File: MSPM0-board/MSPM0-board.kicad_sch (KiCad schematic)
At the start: 30 parts, among them J1 USB_C_Receptacle_USB2.0_16P, J2 TC2030, U1 SPX3819M5-L-3-3, U3 CH340E, U4 LIS2DH, U5 MSPM0G3507SPTR, X1 8MHz

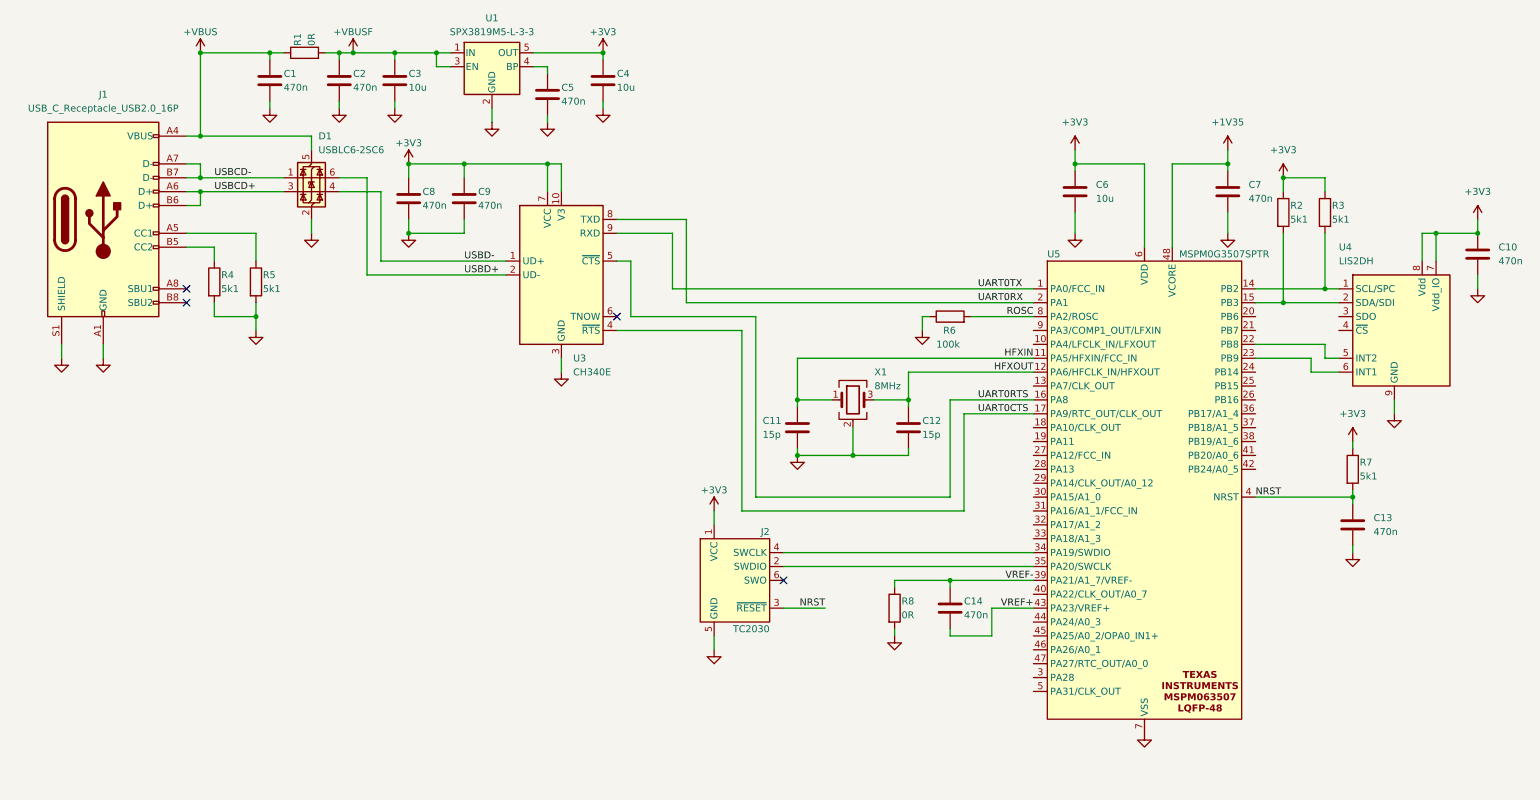
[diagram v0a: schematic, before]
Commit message: mspm0(feat): clean the schematic and generate outputs
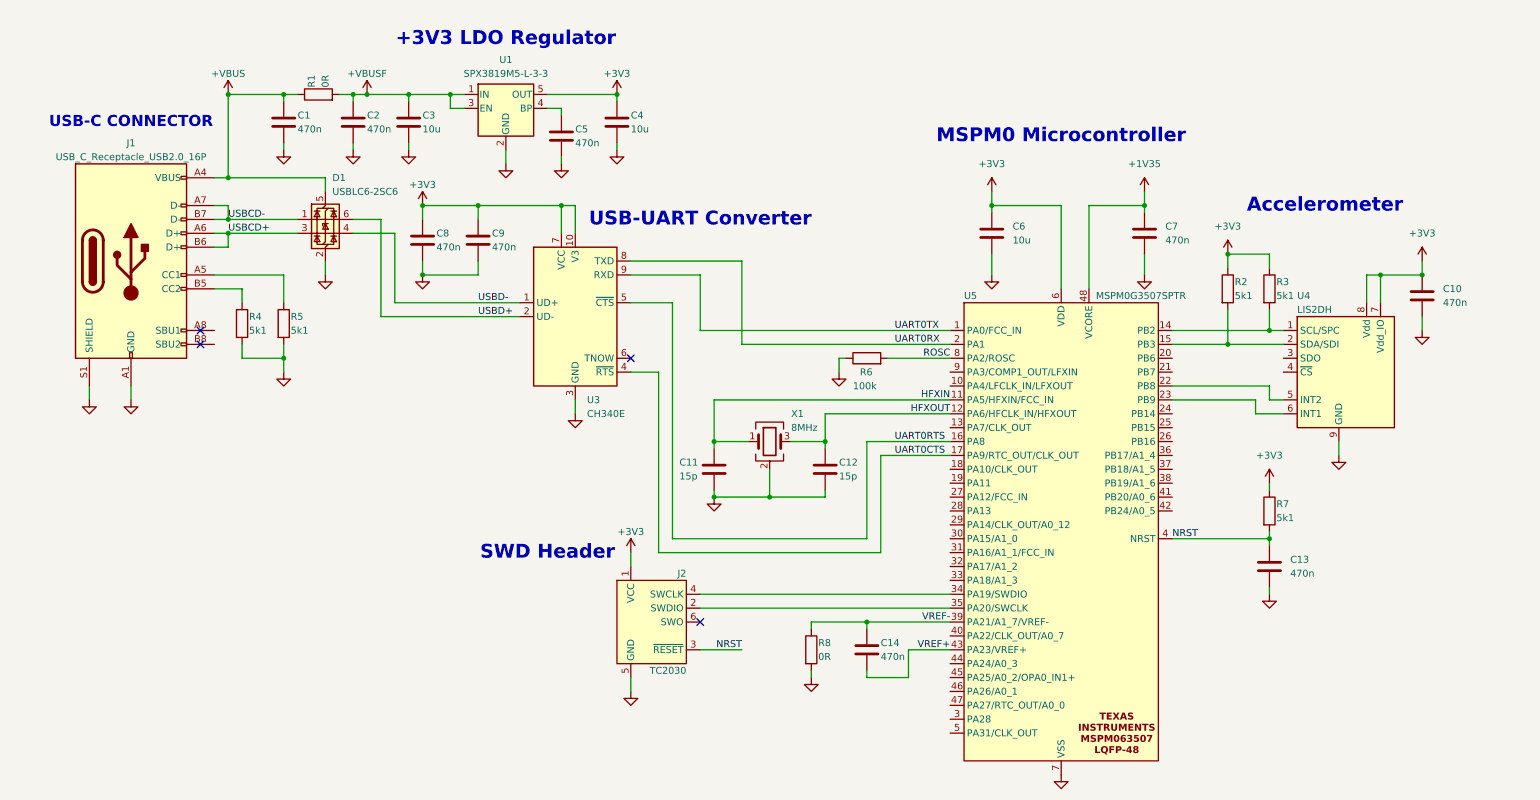
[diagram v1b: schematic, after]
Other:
- note added: "+3V3 LDO Regulator"
- note added: "Accelerometer"
- note added: "MSPM0 Microcontroller"
- note added: "SWD Header"
- note added: "USB-C CONNECTOR"
- note added: "USB-UART Converter"
- moved on the sheet: C1, C10, C11, C12, C13, C14, C2, C3, C4, C5, C6, C7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
